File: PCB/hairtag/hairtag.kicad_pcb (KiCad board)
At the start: 2 copper layers, 24 x 24 mm, 17 parts, among them J1 Flash, J2 BAT, U1 ESP32-C3FH4, X1 XL2EL89CPI-111YLC-40M

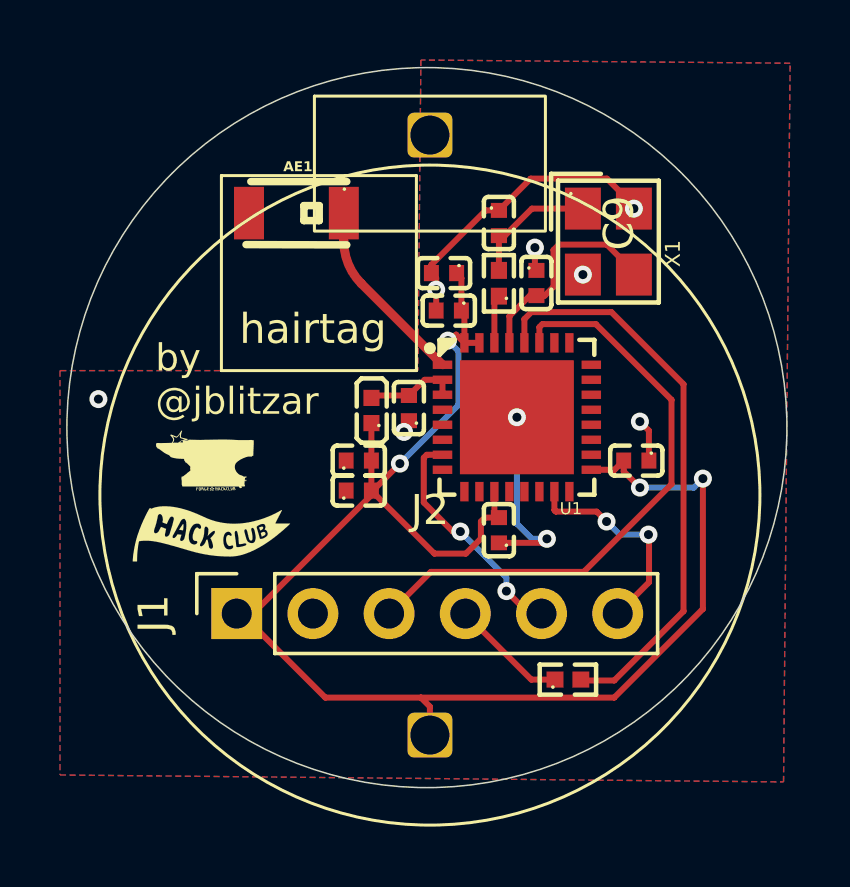
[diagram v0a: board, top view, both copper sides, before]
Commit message: stuff
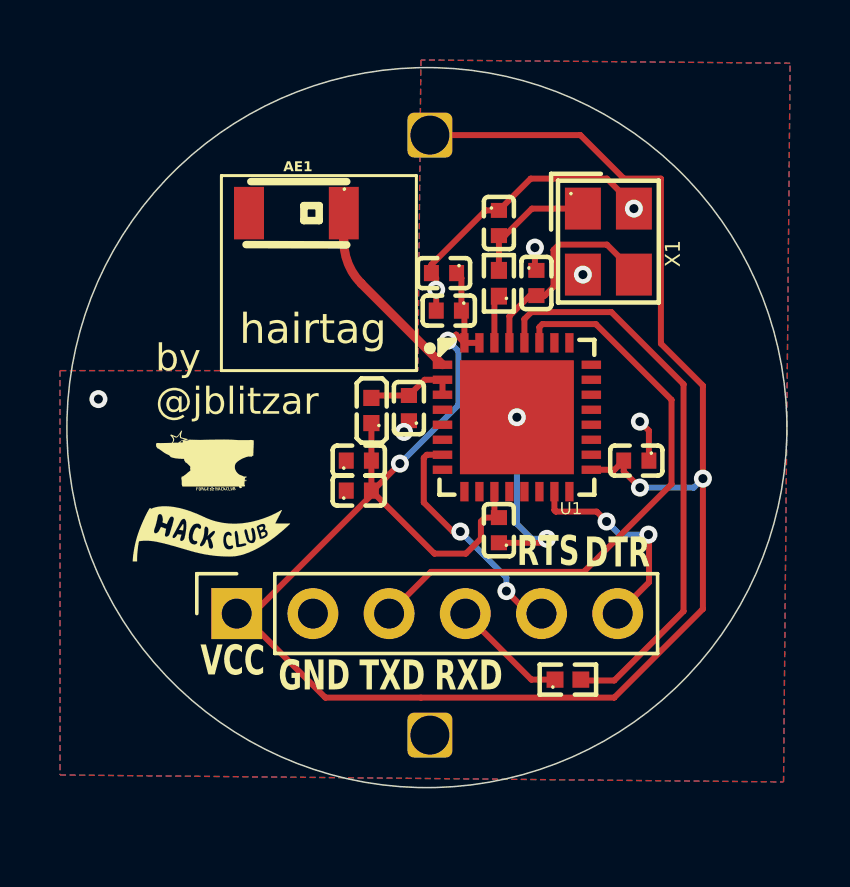
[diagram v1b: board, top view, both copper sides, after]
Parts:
- J2: moved to B.Cu
- turned J2 to 180 degrees
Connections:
- net /CTS renamed /DTR
- J2 pad 1: /VCC -> GND
- J2 pad 2: GND -> /VCC
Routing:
- net /VCC: track 52.5 -> 70.0 mm
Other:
- board text added: "DTR"
- board text added: "GND"
- board text added: "RTS"
- board text added: "RXD"
- board text added: "TXD"
- board text added: "VCC"
